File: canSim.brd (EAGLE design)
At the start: 98.7 x 87.6 mm, 16 parts

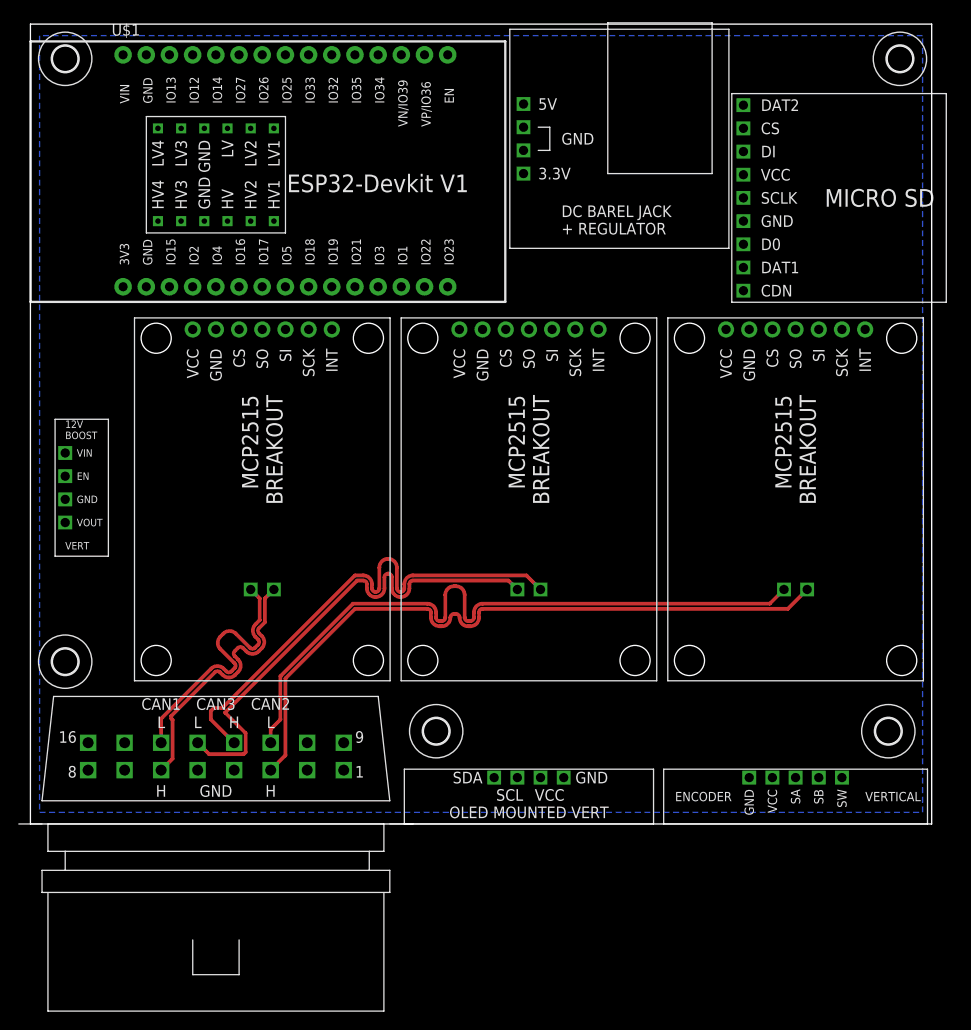
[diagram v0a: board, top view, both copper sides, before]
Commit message: New revision with new OBD-2.  Auto PCB routing to still change.
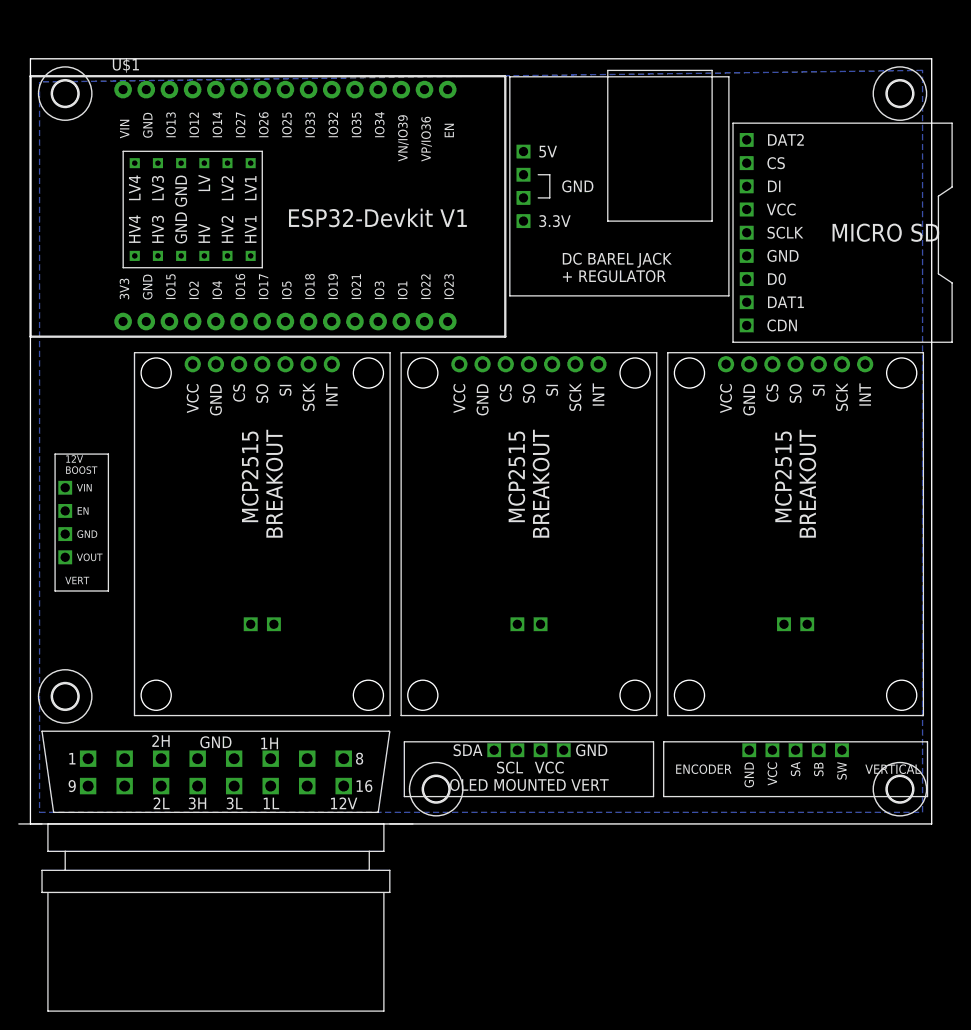
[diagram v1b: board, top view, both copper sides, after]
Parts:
- U$9: value OBD_2FEMALE -> OBD_2FEMALEOBD2_FEMALE_PTH
- moved U$2 58.5 mm to (83.8, 31.8)
- moved U$3 58.5 mm to (25.4, 31.8)
- moved U$8 15.3 mm to (101.0, 64.8)
- moved H2 6.48 mm to (95.2, 3.81)
- moved H3 6.35 mm to (44.5, 3.81)
- moved U$11 5.21 mm to (64.5, 69.8)
- moved U$5 4.58 mm to (16.5, 67.3)
- moved U$1 3.81 mm to (26.7, 67.3)
- moved U$4 3.81 mm to (54.6, 31.8)
- moved H5 3.81 mm to (3.81, 14.0)
- moved U$6 3.81 mm to (2.54, 33.0)
- moved H1 3.81 mm to (95.2, 80.0)
- moved H4 3.81 mm to (3.81, 80.0)
- moved U$10 3.00 mm to (83.8, 3.00)
- moved U$7 3.00 mm to (54.6, 3.00)
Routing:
- net CAN2_P: track 75.3 -> 0.00 mm
- net CAN2_N: track 75.2 -> 0.00 mm
- net CAN3_N: track 55.2 -> 0.00 mm
- net CAN3_P: track 55.2 -> 0.00 mm
- net CAN1_P: track 29.2 -> 0.00 mm
- net CAN1_N: track 29.2 -> 0.00 mm
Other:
- board size 98.7 x 87.6 mm -> 98.7 x 83.8 mm
